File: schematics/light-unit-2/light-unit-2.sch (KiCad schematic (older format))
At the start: 8 parts

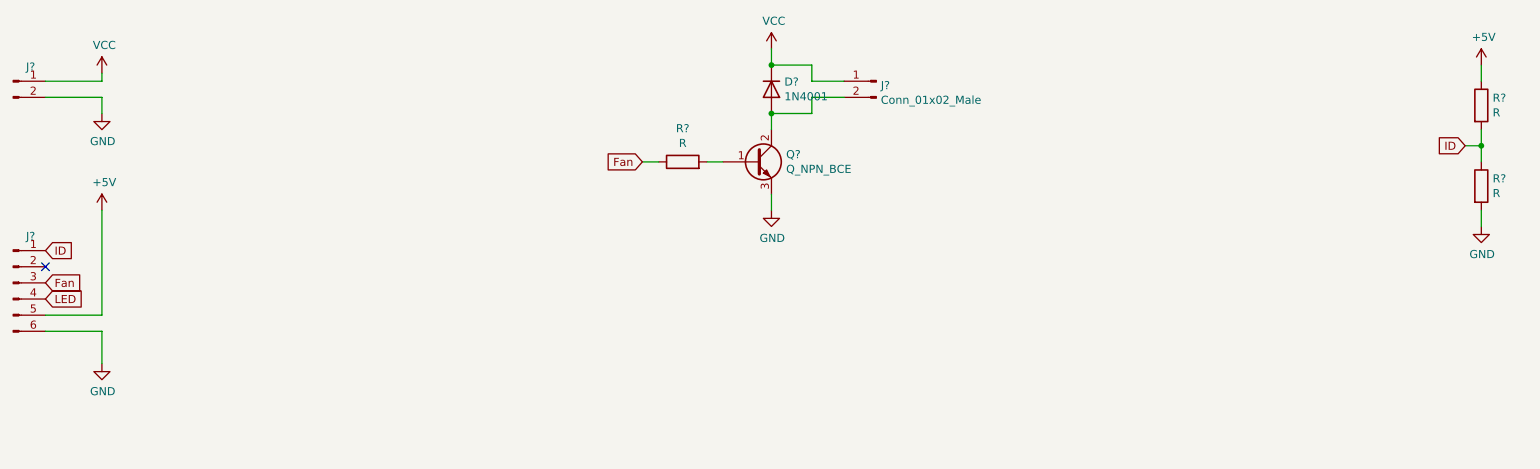
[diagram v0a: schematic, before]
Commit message: Complete Light Unit 2
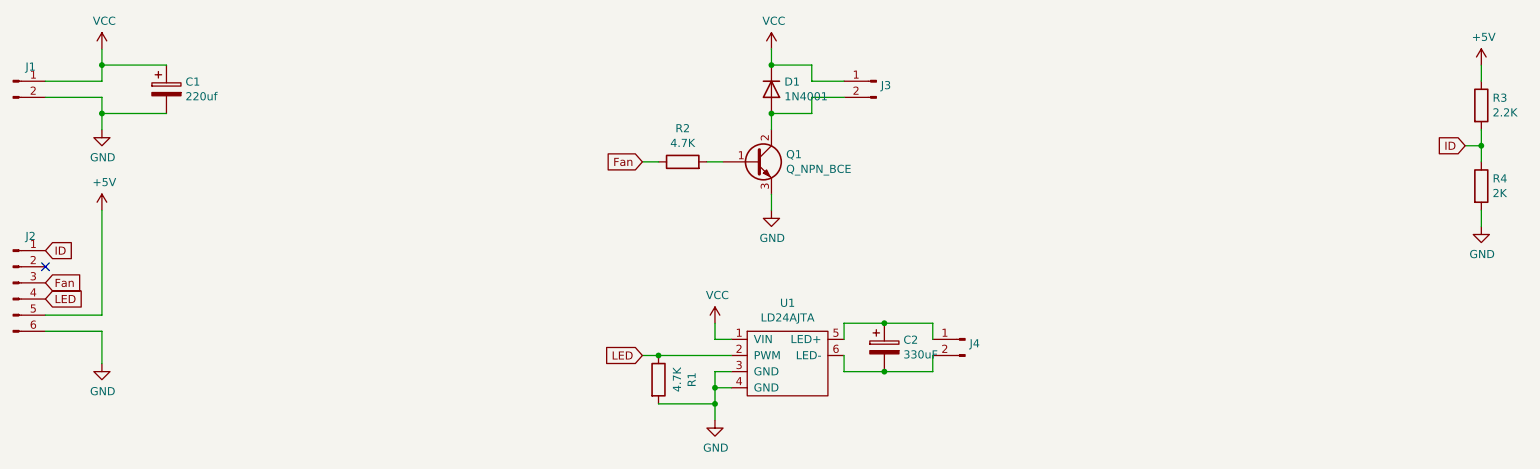
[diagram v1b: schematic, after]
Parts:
- added C1: 220uf, symbol Device:CP
- added C2: 330uF, symbol Device:CP
- added J4: Conn_01x02_Male, symbol Connector:Conn_01x02_Male
- added R1: 4.7K, symbol Device:R
- added U1: LD24AJTA, symbol light-unit-2-library:LD24AJTA
- R2: renamed from R?; value R -> 4.7K
- R3: renamed from R?; value R -> 2.2K
- R4: renamed from R?; value R -> 2K
- gave numbers to parts that had none: 5
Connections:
- net GND: now also C1.2, R1.2, U1.3 (GND), U1.4 (GND)
- net LED: now also R1.1, U1.2 (PWM)
- net VCC: now also C1.1, U1.1 (VIN)
- new net: C2.1, J4.1 (Pin_1), U1.5 (LED+)
- new net: C2.2, J4.2 (Pin_2), U1.6 (LED-)
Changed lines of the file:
@@
 $EndDescr
 $Comp
-L power:VCC #PWR?
+L power:VCC #PWR01
 U 1 1 64D30CF8
-P 1800 950
-F 0 "#PWR?" H 1800 800 50  0001 C CNN
-F 1 "VCC" H 1815 1123 50  0000 C CNN
-F 2 "" H 1800 950 50  0001 C CNN
-F 3 "" H 1800 950 50  0001 C CNN
-	1    1800 950
-	1    0    0    -1
-$EndComp
-$Comp
-L power:GND #PWR?
+P 1800 800
+F 0 "#PWR01" H 1800 650 50  0001 C CNN
+F 1 "VCC" H 1815 973 50  0000 C CNN
+F 2 "" H 1800 800 50  0001 C CNN
+F 3 "" H 1800 800 50  0001 C CNN
+	1    1800 800
+	1    0    0    -1
+$EndComp
+$Comp
+L power:GND #PWR02
 U 1 1 64D30E73
-P 1800 1200
-F 0 "#PWR?" H 1800 950 50  0001 C CNN
-F 1 "GND" H 1805 1027 50  0000 C CNN
-F 2 "" H 1800 1200 50  0001 C CNN
-F 3 "" H 1800 1200 50  0001 C CNN
-	1    1800 1200
-	1    0    0    -1
-$EndComp
-$Comp
-L Connector:Conn_01x02_Male J?
+P 1800 1300
+F 0 "#PWR02" H 1800 1050 50  0001 C CNN
+F 1 "GND" H 1805 1127 50  0000 C CNN
+F 2 "" H 1800 1300 50  0001 C CNN
+F 3 "" H 1800 1300 50  0001 C CNN
+	1    1800 1300
+	1    0    0    -1
+$EndComp
+$Comp
+L Connector:Conn_01x02_Male J1
 U 1 1 64D315FC
 P 1250 1000
-F 0 "J?" H 1358 1089 50  0000 C CNN
+F 0 "J1" H 1358 1089 50  0000 C CNN
 F 1 "Conn_01x02_Male" H 1358 1090 50  0001 C CNN
 F 2 "" H 1250 1000 50  0001 C CNN
@@
 	1450 1000 1800 1000
 Wire Wire Line
-	1800 1000 1800 950
-Wire Wire Line
 	1450 1100 1800 1100
 Wire Wire Line
 	1800 1100 1800 1200
 $Comp
-L Connector:Conn_01x06_Male J?
+L Connector:Conn_01x06_Male J2
 U 1 1 64D3266B
 P 1250 2250
-F 0 "J?" H 1358 2539 50  0000 C CNN
+F 0 "J2" H 1358 2539 50  0000 C CNN
 F 1 "Conn_01x06_Male" H 1358 2540 50  0001 C CNN
 F 2 "" H 1250 2250 50  0001 C CNN
@@
 $EndComp
 $Comp
-L power:+5V #PWR?
+L power:+5V #PWR03
 U 1 1 64D33754
 P 1800 1800
-F 0 "#PWR?" H 1800 1650 50  0001 C CNN
+F 0 "#PWR03" H 1800 1650 50  0001 C CNN
 F 1 "+5V" H 1815 1973 50  0000 C CNN
 F 2 "" H 1800 1800 50  0001 C CNN
@@
 $EndComp
 $Comp
-L power:GND #PWR?
+L power:GND #PWR04
 U 1 1 64D348EB
 P 1800 2750
-F 0 "#PWR?" H 1800 2500 50  0001 C CNN
+F 0 "#PWR04" H 1800 2500 50  0001 C CNN
 F 1 "GND" H 1805 2577 50  0000 C CNN
 F 2 "" H 1800 2750 50  0001 C CNN
@@
 ID
 $Comp
-L Device:R R?
+L Device:R R3
 U 1 1 64D358BA
 P 10350 1150
-F 0 "R?" H 10420 1196 50  0000 L CNN
-F 1 "R" H 10420 1105 50  0000 L CNN
+F 0 "R3" H 10420 1196 50  0000 L CNN
+F 1 "2.2K" H 10420 1105 50  0000 L CNN
 F 2 "" V 10280 1150 50  0001 C CNN
 F 3 "~" H 10350 1150 50  0001 C CNN
@@
 $EndComp
 $Comp
-L power:+5V #PWR?
+L power:+5V #PWR09
 U 1 1 64D36410
 P 10350 900
-F 0 "#PWR?" H 10350 750 50  0001 C CNN
+F 0 "#PWR09" H 10350 750 50  0001 C CNN
 F 1 "+5V" H 10365 1073 50  0000 C CNN
 F 2 "" H 10350 900 50  0001 C CNN
@@
 $EndComp
 $Comp
-L Device:R R?
+L Device:R R4
 U 1 1 64D370A1
 P 10350 1650
-F 0 "R?" H 10420 1696 50  0000 L CNN
-F 1 "R" H 10420 1605 50  0000 L CNN
+F 0 "R4" H 10420 1696 50  0000 L CNN
+F 1 "2K" H 10420 1605 50  0000 L CNN
 F 2 "" V 10280 1650 50  0001 C CNN
 F 3 "~" H 10350 1650 50  0001 C CNN
@@
 $EndComp
 $Comp
-L power:GND #PWR?
+L power:GND #PWR010
 U 1 1 64D37199
 P 10350 1900
-F 0 "#PWR?" H 10350 1650 50  0001 C CNN
+F 0 "#PWR010" H 10350 1650 50  0001 C CNN
 F 1 "GND" H 10355 1727 50  0000 C CNN
 F 2 "" H 10350 1900 50  0001 C CNN
@@
 	10350 1000 10350 900
 $Comp
-L Connector:Conn_01x02_Male J?
+L Connector:Conn_01x02_Male J3
 U 1 1 64D3BB1E
 P 6600 1000
-F 0 "J?" H 6572 974 50  0000 R CNN
-F 1 "Conn_01x02_Male" H 6572 883 50  0000 R CNN
+F 0 "J3" H 6572 974 50  0000 R CNN
+F 1 "Conn_01x02_Male" H 6572 883 50  0001 R CNN
 F 2 "" H 6600 1000 50  0001 C CNN
 F 3 "~" H 6600 1000 50  0001 C CNN
@@
 $EndComp
 $Comp
-L power:VCC #PWR?
+L power:VCC #PWR07
 U 1 1 64D3C534
 P 5950 800
-F 0 "#PWR?" H 5950 650 50  0001 C CNN
+F 0 "#PWR07" H 5950 650 50  0001 C CNN
 F 1 "VCC" H 5965 973 50  0000 C CNN
 F 2 "" H 5950 800 50  0001 C CNN
@@
 $EndComp
 $Comp
-L power:GND #PWR?
+L power:GND #PWR08
 U 1 1 64D3D34D
 P 5950 1800
-F 0 "#PWR?" H 5950 1550 50  0001 C CNN
+F 0 "#PWR08" H 5950 1550 50  0001 C CNN
 F 1 "GND" H 5955 1627 50  0000 C CNN
 F 2 "" H 5950 1800 50  0001 C CNN
@@
 Fan
 $Comp
-L Device:R R?
+L Device:R R2
 U 1 1 64D3D73F
 P 5400 1500
-F 0 "R?" V 5607 1500 50  0000 C CNN
-F 1 "R" V 5516 1500 50  0000 C CNN
+F 0 "R2" V 5607 1500 50  0000 C CNN
+F 1 "4.7K" V 5516 1500 50  0000 C CNN
 F 2 "" V 5330 1500 50  0001 C CNN
 F 3 "~" H 5400 1500 50  0001 C CNN
@@
 $EndComp
 $Comp
-L Device:Q_NPN_BCE Q?
+L Device:Q_NPN_BCE Q1
 U 1 1 64D40B66
 P 5850 1500
-F 0 "Q?" H 6041 1546 50  0000 L CNN
+F 0 "Q1" H 6041 1546 50  0000 L CNN
 F 1 "Q_NPN_BCE" H 6041 1455 50  0000 L CNN
 F 2 "" H 6050 1600 50  0001 C CNN
@@
 	5950 1700 5950 1800
 $Comp
-L Diode:1N4001 D?
+L Diode:1N4001 D1
 U 1 1 64D4310A
 P 5950 1050
-F 0 "D?" V 5904 1130 50  0000 L CNN
+F 0 "D1" V 5904 1130 50  0000 L CNN
 F 1 "1N4001" V 5995 1130 50  0000 L CNN
 F 2 "Diode_THT:D_DO-41_SOD81_P10.16mm_Horizontal" H 5950 875 50  0001 C CNN
@@
 	6200 1100 6400 1100
 Connection ~ 5950 1200
+$Comp
+L Connector:Conn_01x02_Male J4
+U 1 1 64D33418
+P 7150 2600
+F 0 "J4" H 7122 2574 50  0000 R CNN
+F 1 "Conn_01x02_Male" H 7122 2483 50  0001 R CNN
+F 2 "" H 7150 2600 50  0001 C CNN
+F 3 "~" H 7150 2600 50  0001 C CNN
+	1    7150 2600
+	-1   0    0    -1
+$EndComp
+$Comp
+L power:VCC #PWR05
+U 1 1 64D3341E
+P 5600 2500
+F 0 "#PWR05" H 5600 2350 50  0001 C CNN
+F 1 "VCC" H 5615 2673 50  0000 C CNN
+F 2 "" H 5600 2500 50  0001 C CNN
+F 3 "" H 5600 2500 50  0001 C CNN
+	1    5600 2500
+	1    0    0    -1
+$EndComp
+$Comp
+L power:GND #PWR06
+U 1 1 64D33424
+P 5600 3100
+F 0 "#PWR06" H 5600 2850 50  0001 C CNN
+F 1 "GND" H 5605 2927 50  0000 C CNN
+F 2 "" H 5600 3100 50  0001 C CNN
+F 3 "" H 5600 3100 50  0001 C CNN
+	1    5600 3100
+	1    0    0    -1
+$EndComp
+Text GLabel 5150 2700 0    50   Input ~ 0
+LED
+$Comp
+L Device:R R1
+U 1 1 64D3342B
+P 5250 2850
+F 0 "R1" V 5457 2850 50  0000 C CNN
+F 1 "4.7K" V 5366 2850 50  0000 C CNN
+F 2 "" V 5180 2850 50  0001 C CNN
+F 3 "~" H 5250 2850 50  0001 C CNN
+	1    5250 2850
+	1    0    0    -1
+$EndComp
+Wire Wire Line
+	5150 2700 5250 2700
+$Comp
+L Device:CP C1
+U 1 1 64D346E8
+P 2200 1050
+F 0 "C1" H 2318 1096 50  0000 L CNN
+F 1 "220uf" H 2318 1005 50  0000 L CNN
+F 2 "" H 2238 900 50  0001 C CNN
+F 3 "~" H 2200 1050 50  0001 C CNN
+	1    2200 1050
+	1    0    0    -1
+$EndComp
+Wire Wire Line
+	2200 900  1800 900
+Wire Wire Line
+	1800 900  1800 1000
+Wire Wire Line
+	1800 900  1800 800
+Connection ~ 1800 900
+Wire Wire Line
+	2200 1200 1800 1200
+Wire Wire Line
+	1800 1300 1800 1200
+Connection ~ 1800 1200
+$Comp
+L light-unit-2-library:LD24AJTA U1
+U 1 1 64D3CF2D
+P 6050 2500
+F 0 "U1" H 6050 2625 50  0000 C CNN
+F 1 "LD24AJTA" H 6050 2534 50  0000 C CNN
+F 2 "" H 6050 2650 50  0001 C CNN
+F 3 "" H 6050 2650 50  0001 C CNN
+	1    6050 2500
+	1    0    0    -1
+$EndComp
+Wire Wire Line
+	5700 2800 5600 2800
+Wire Wire Line
+	5600 2800 5600 2900
+Wire Wire Line
+	5700 2900 5600 2900
+Connection ~ 5600 2900
+Wire Wire Line
+	5600 2900 5600 3000
+$Comp
+L Device:CP C2
+U 1 1 64D41E3F
+P 6650 2650
+F 0 "C2" H 6768 2696 50  0000 L CNN
+F 1 "330uF" H 6768 2605 50  0000 L CNN
+F 2 "" H 6688 2500 50  0001 C CNN
+F 3 "~" H 6650 2650 50  0001 C CNN
+	1    6650 2650
+	1    0    0    -1
+$EndComp
+Wire Wire Line
+	6950 2600 6950 2500
+Wire Wire Line
+	6950 2500 6650 2500
+Wire Wire Line
+	6650 2500 6400 2500
+Wire Wire Line
+	6400 2500 6400 2600
+Connection ~ 6650 2500
+Wire Wire Line
+	6400 2700 6400 2800
+Wire Wire Line
+	6400 2800 6650 2800
+Wire Wire Line
+	6950 2700 6950 2800
+Wire Wire Line
+	6950 2800 6650 2800
+Connection ~ 6650 2800
+Wire Wire Line
+	5250 2700 5700 2700
+Connection ~ 5250 2700
+Wire Wire Line
+	5250 3000 5600 3000
+Connection ~ 5600 3000
+Wire Wire Line
+	5600 3000 5600 3100
+Wire Wire Line
+	5700 2600 5600 2600
+Wire Wire Line
+	5600 2600 5600 2500
 $EndSCHEMATC
